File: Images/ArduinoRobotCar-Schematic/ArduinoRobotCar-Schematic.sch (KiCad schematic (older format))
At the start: 12 parts

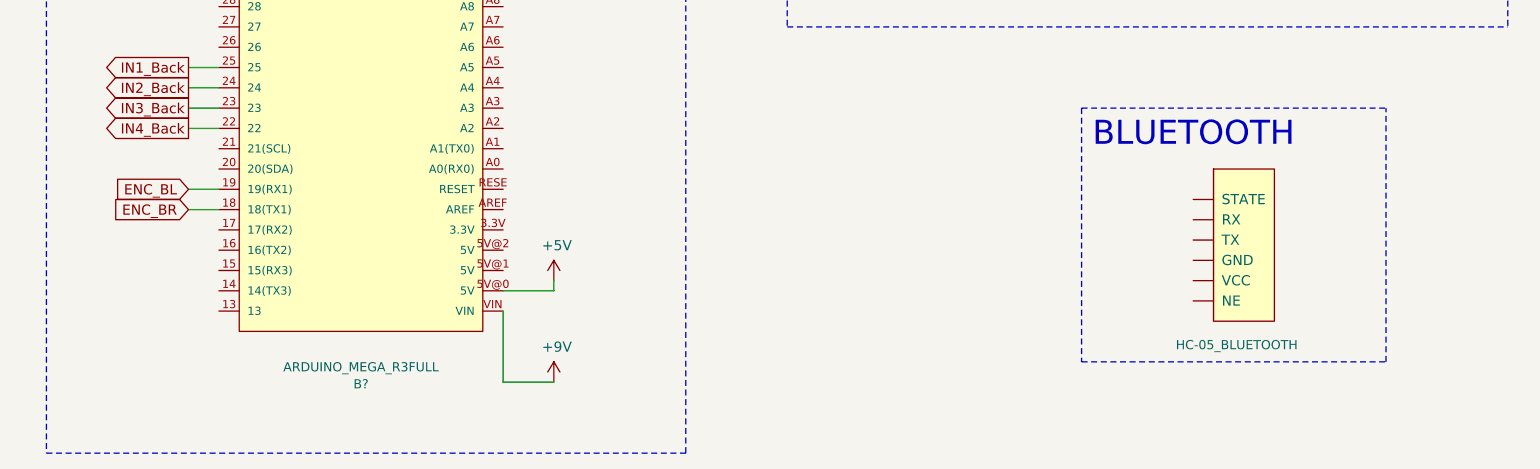
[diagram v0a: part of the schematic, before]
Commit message: Update schematic
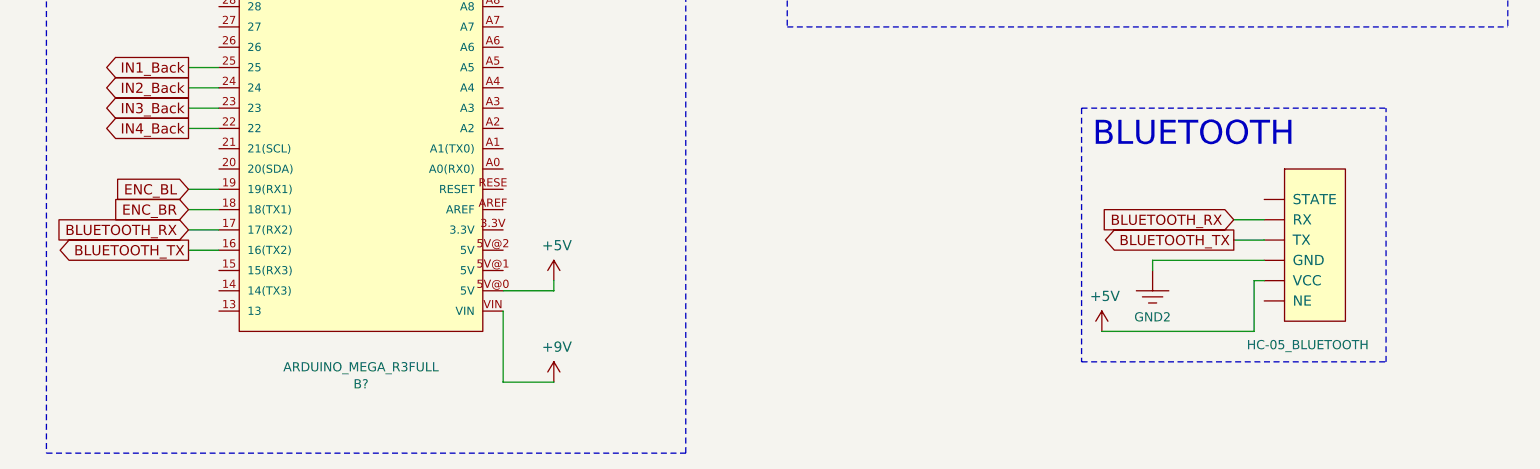
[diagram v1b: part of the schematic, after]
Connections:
- net +5V: now also J?.~ (VCC)
- net 3.3V: now also J?.~ (VCC)
- net BLUETOOTH_TX: now reaches B?.16 (16(TX2))
- net BLUETOOTH_TX: now also J?.~ (VCC)
- net BLUETOOTH_RX: now reaches B?.17 (17(RX2))
- net BLUETOOTH_RX: now also J?.~ (VCC)
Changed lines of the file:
@@
 L AA_Custom_Components:HC-05_BLUETOOTH J?
 U 1 1 61E112FB
-P 6900 5900
-F 0 "J?" H 7328 5967 45  0001 L CNN
-F 1 "HC-05_BLUETOOTH" H 6564 5383 45  0000 L CNN
-F 2 "" H 7050 6200 20  0001 C CNN
-F 3 "" H 6300 5500 50  0001 C CNN
-	1    6900 5900
+P 7250 5900
+F 0 "J?" H 7678 5967 45  0001 L CNN
+F 1 "HC-05_BLUETOOTH" H 6914 5383 45  0000 L CNN
+F 2 "" H 7400 6200 20  0001 C CNN
+F 3 "" H 6650 5500 50  0001 C CNN
+	1    7250 5900
 	1    0    0    -1
 $EndComp
+$Comp
+L power:+5V #PWR?
+U 1 1 61E51311
+P 6200 6350
+F 0 "#PWR?" H 6200 6200 50  0001 C CNN
+F 1 "+5V" H 6215 6523 50  0000 C CNN
+F 2 "" H 6200 6350 50  0001 C CNN
+F 3 "" H 6200 6350 50  0001 C CNN
+	1    6200 6350
+	1    0    0    -1
+$EndComp
+Text GLabel 1700 5850 0    50   Input ~ 0
+BLUETOOTH_RX
+Text GLabel 1700 5950 0    50   Output ~ 0
+BLUETOOTH_TX
+Wire Wire Line
+	1700 5850 1850 5850
+Wire Wire Line
+	1700 5950 1850 5950
+Text GLabel 6850 5800 0    50   Input ~ 0
+BLUETOOTH_RX
+Text GLabel 6850 5900 0    50   Output ~ 0
+BLUETOOTH_TX
+Wire Wire Line
+	6850 5800 7000 5800
+Wire Wire Line
+	6850 5900 7000 5900
+Wire Wire Line
+	6200 6350 6950 6350
+Wire Wire Line
+	6950 6350 6950 6100
+Wire Wire Line
+	6950 6100 7000 6100
+$Comp
+L SparkFun-PowerSymbols:GND2 #GND?
+U 1 1 61E6A065
+P 6450 6050
+F 0 "#GND?" H 6500 6000 45  0001 L BNN
+F 1 "GND2" H 6450 5820 45  0000 C CNN
+F 2 "" H 6450 5725 60  0001 C CNN
+F 3 "" H 6450 5950 60  0001 C CNN
+	1    6450 6050
+	1    0    0    -1
+$EndComp
+Wire Wire Line
+	6450 6050 6450 6000
+Wire Wire Line
+	6450 6000 7000 6000
 $EndSCHEMATC
